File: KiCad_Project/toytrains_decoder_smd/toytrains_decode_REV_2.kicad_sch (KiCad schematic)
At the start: 43 parts, among them IC1 LM2596S, IC2 TLE5206-2G, Q10 BSS138, Q11 BSS138, Q12 BSS138, Q7 BSS138, Q8 BSS138, Q9 BSS138

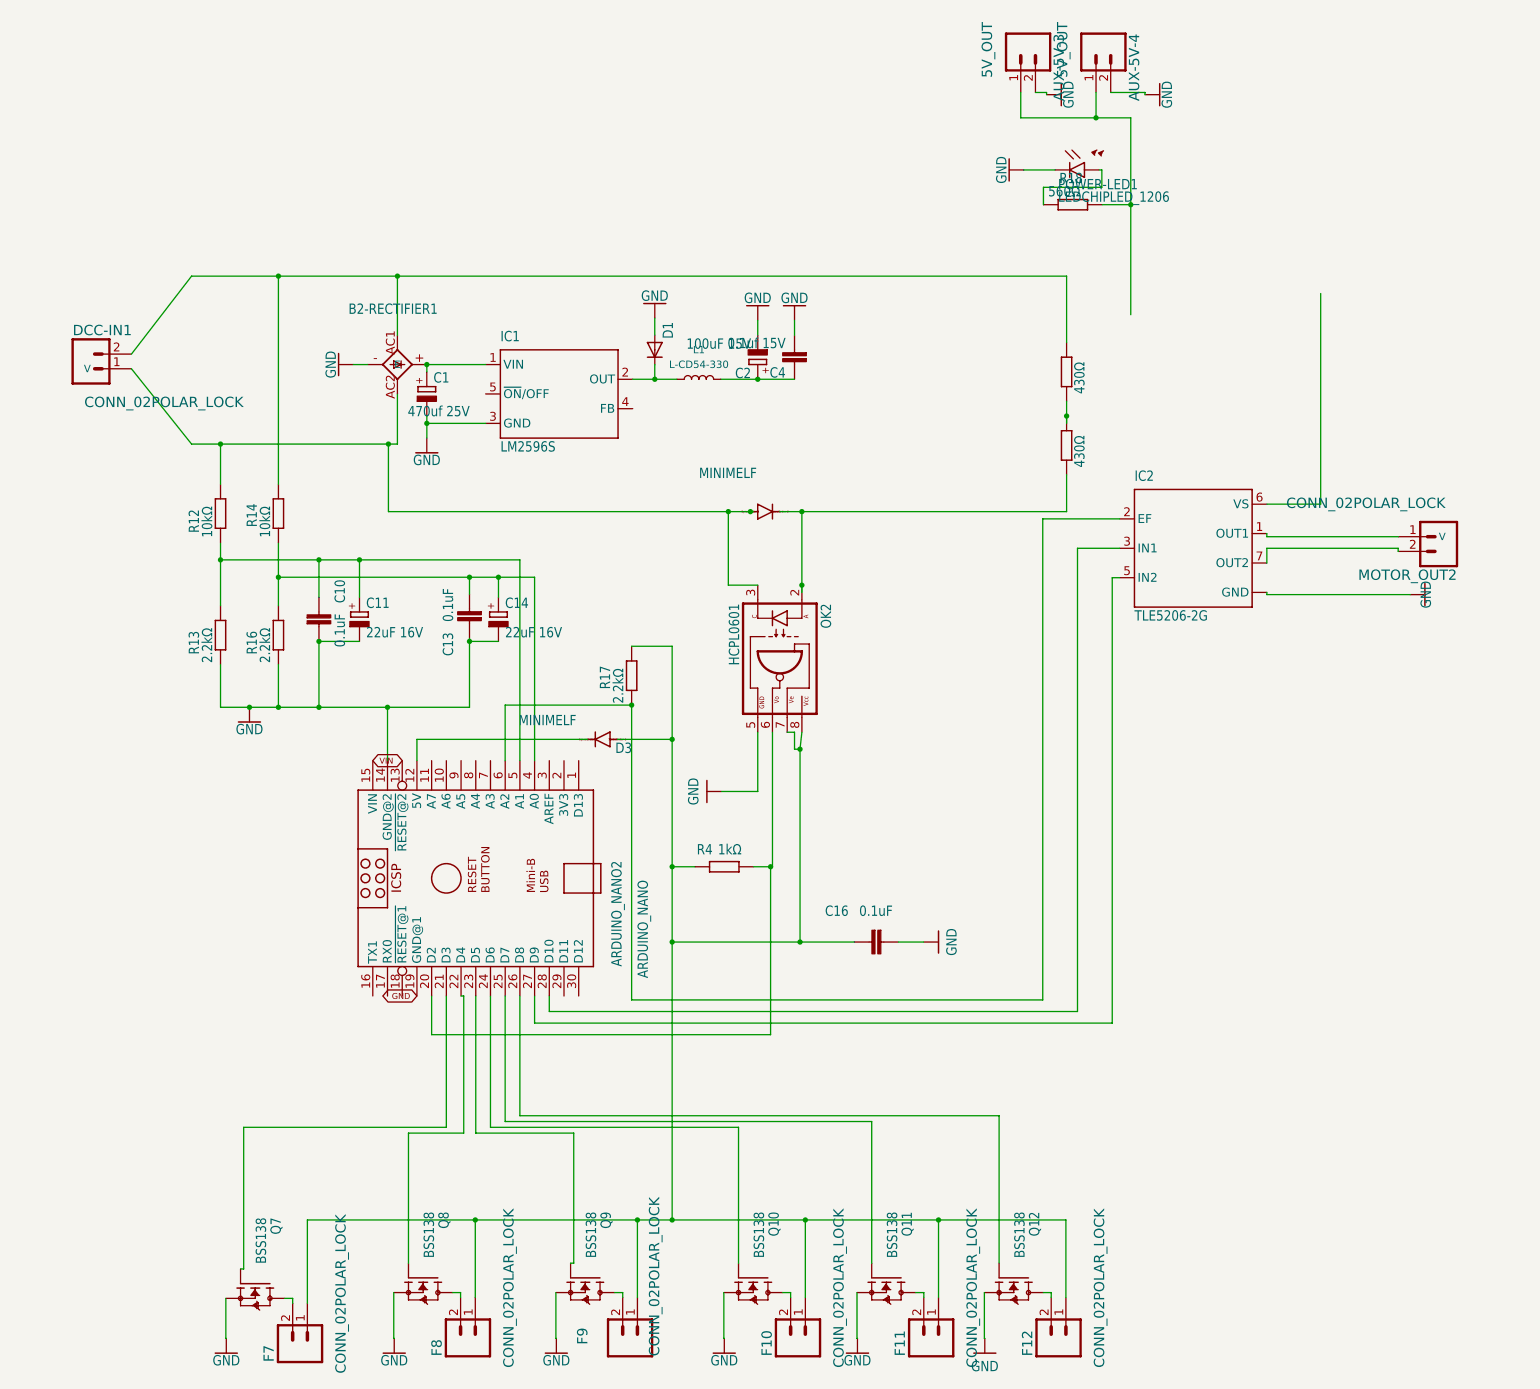
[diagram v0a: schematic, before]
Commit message: esp32_decoder kicad setup
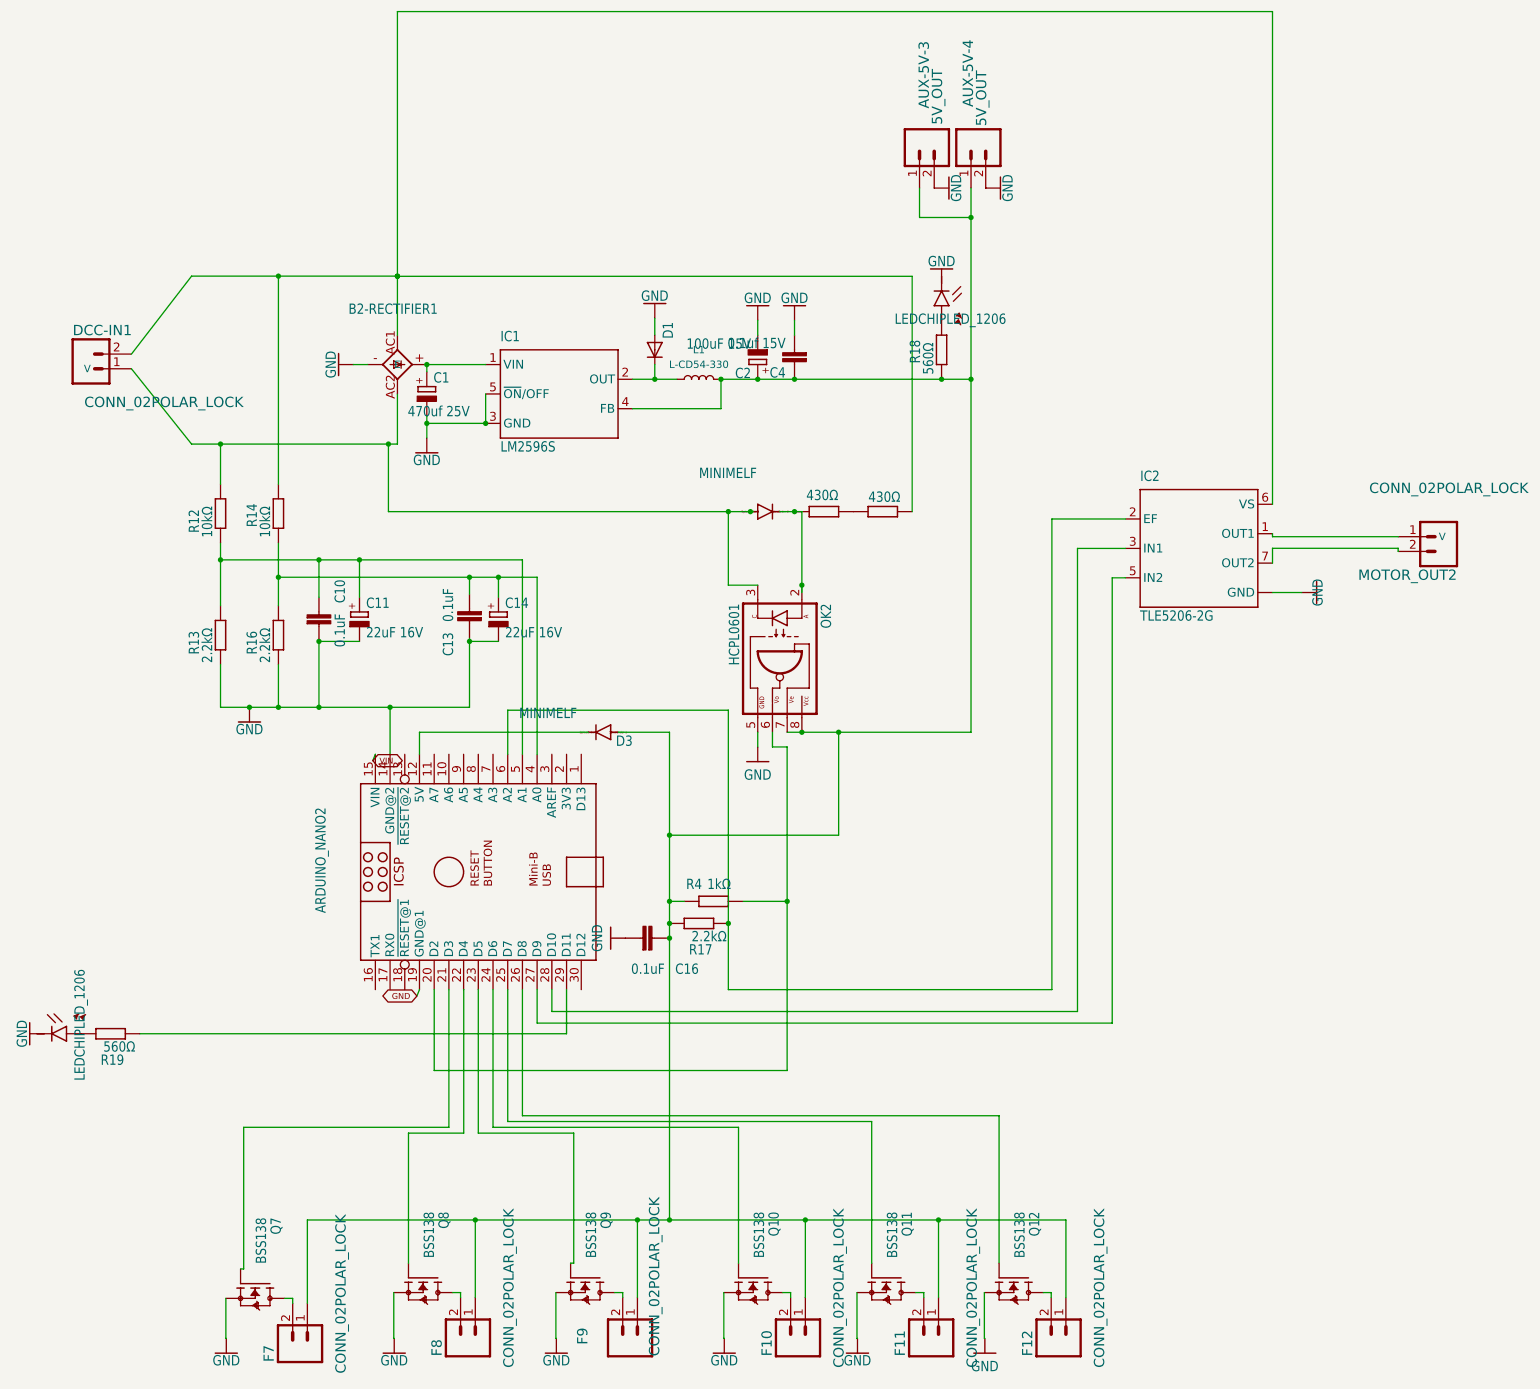
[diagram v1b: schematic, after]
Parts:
- added POWER-LED2: LEDCHIPLED_1206, toytrains_decoder_smd:CHIPLED_1206, symbol toytrains_decoder_smd-eagle-import:led_259_LEDCHIPLED_1206
- added R19: 560Ω, toytrains_decoder_smd:R1206, symbol toytrains_decoder_smd-eagle-import:rcl_334_R-EU_R1206
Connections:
- net GND: now also IC1.5 (~{ON}/OFF); no longer POWER-LED1.C
- net at C16.1, D3.A, F10.1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: now also AUX-5V-3.1, AUX-5V-4.1, C2.+, C4.1, IC1.4 (FB), L1.2, R18.2
- net at ARDUINO_NANO2.29 (D11): now also R19.2
- net at B2-RECTIFIER1.AC1, DCC-IN1.2, R14.1: now also IC2.6 (VS), R5.1; no longer R5.2
- net at R6.2: now also R5.2; no longer R5.1
- net at POWER-LED1.A: now also R18.1; no longer R18.2
- new net: POWER-LED2.A, R19.1
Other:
- moved on the sheet: ARDUINO_NANO2, AUX-5V-3, AUX-5V-4, D3, IC2, R18
